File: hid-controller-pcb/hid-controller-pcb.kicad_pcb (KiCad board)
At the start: 2 copper layers, 16 parts, among them IC1 RT9080-33GJ5, J1 10118194-0011LF, U1 STM32F103C8Tx, U2 32.768KHz, U3 COM-09032, U4 COM-09032, Y1 8MHz

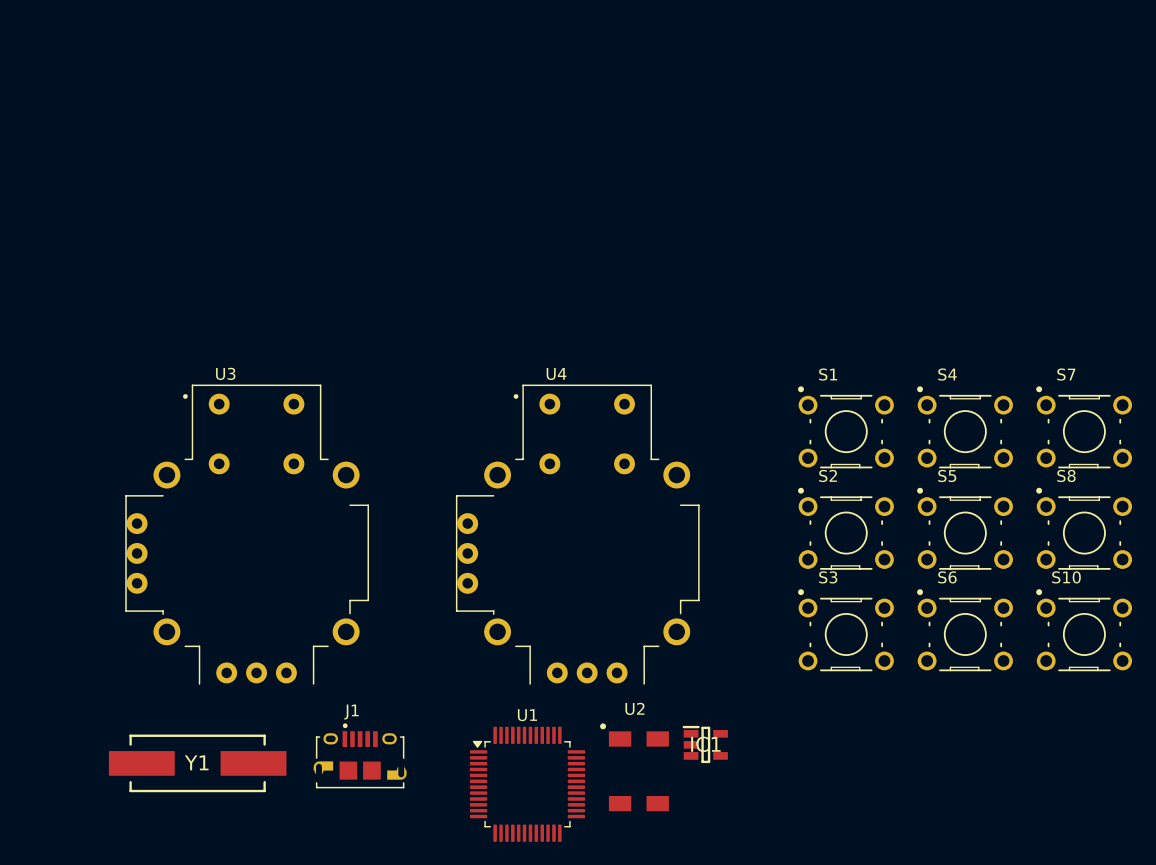
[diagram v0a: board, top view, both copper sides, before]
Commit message: schematic finished? now onto layout
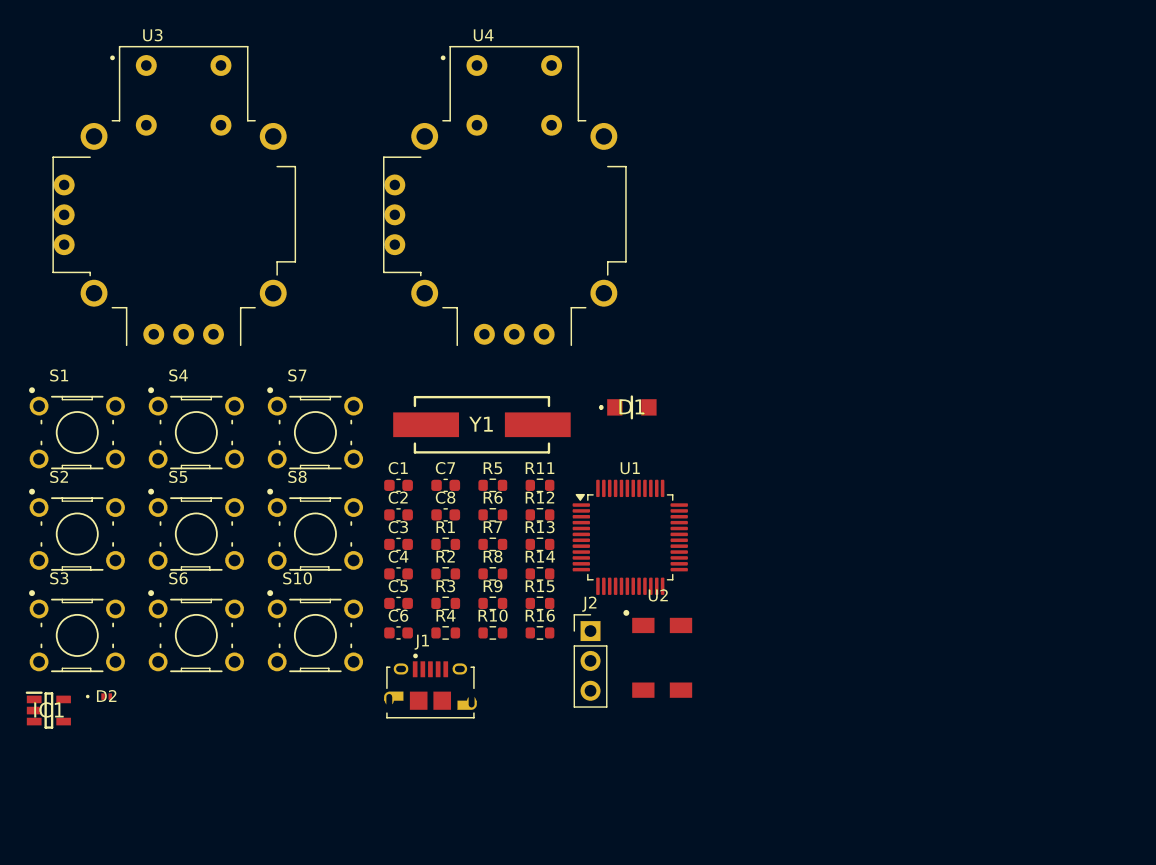
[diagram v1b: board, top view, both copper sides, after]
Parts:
- added C1: 4.7uF, Capacitor_SMD:C_0603_1608Metric, F.Cu at (114.9, 100.6)
- added C2: 26pF, Capacitor_SMD:C_0603_1608Metric, F.Cu at (114.9, 103.1)
- added C3: 26pF, Capacitor_SMD:C_0603_1608Metric, F.Cu at (114.9, 105.7)
- added C4: 8pF, Capacitor_SMD:C_0603_1608Metric, F.Cu at (114.9, 108.2)
- added C5: 8pF, Capacitor_SMD:C_0603_1608Metric, F.Cu at (114.9, 110.7)
- added C6: 0.1uF, Capacitor_SMD:C_0603_1608Metric, F.Cu at (114.9, 113.2)
- added C7: 0.1uF, Capacitor_SMD:C_0603_1608Metric, F.Cu at (118.9, 100.6)
- added C8: 2.2uF, Capacitor_SMD:C_0603_1608Metric, F.Cu at (118.9, 103.1)
- added D1: 3.4V, lib:SMFA2005CA, F.Cu at (134.7, 94.0)
- added D2: 6V, lib:DIODE_VESD05A1B-HD1-GS08_VIS, F.Cu at (90.1, 118.6)
- added J2: Jumper, Connector_PinHeader_2.54mm:PinHeader_1x03_P2.54mm_Vertical, F.Cu at (131.2, 113.0)
- added R1: 22R, Resistor_SMD:R_0603_1608Metric, F.Cu at (118.9, 105.7)
- added R10: 20kR, Resistor_SMD:R_0603_1608Metric, F.Cu at (122.9, 113.2)
- added R11: 20kR, Resistor_SMD:R_0603_1608Metric, F.Cu at (126.9, 100.6)
- added R12: 20kR, Resistor_SMD:R_0603_1608Metric, F.Cu at (126.9, 103.1)
- added R13: 20kR, Resistor_SMD:R_0603_1608Metric, F.Cu at (126.9, 105.7)
- added R14: 20kR, Resistor_SMD:R_0603_1608Metric, F.Cu at (126.9, 108.2)
- added R15: 20kR, Resistor_SMD:R_0603_1608Metric, F.Cu at (126.9, 110.7)
- added R16: 20kR, Resistor_SMD:R_0603_1608Metric, F.Cu at (126.9, 113.2)
- added R2: 22R, Resistor_SMD:R_0603_1608Metric, F.Cu at (118.9, 108.2)
- added R3: 1.5kR, Resistor_SMD:R_0603_1608Metric, F.Cu at (118.9, 110.7)
- added R4: 1.5kR, Resistor_SMD:R_0603_1608Metric, F.Cu at (118.9, 113.2)
- added R5: 68kR, Resistor_SMD:R_0603_1608Metric, F.Cu at (122.9, 100.6)
- added R6: 13kR, Resistor_SMD:R_0603_1608Metric, F.Cu at (122.9, 103.1)
- added R7: 1.5kR, Resistor_SMD:R_0603_1608Metric, F.Cu at (122.9, 105.7)
- added R8: 1.5kR, Resistor_SMD:R_0603_1608Metric, F.Cu at (122.9, 108.2)
- added R9: 20kR, Resistor_SMD:R_0603_1608Metric, F.Cu at (122.9, 110.7)
- moved S1 65.4 mm to (87.6, 96.1)
- moved S10 65.4 mm to (107.8, 113.4)
- moved S2 65.4 mm to (87.6, 104.8)
- moved S3 65.4 mm to (87.6, 113.4)
- moved S7 65.4 mm to (107.8, 96.1)
- moved S8 65.4 mm to (107.8, 104.8)
- moved S4 65.4 mm to (97.7, 96.1)
- moved S5 65.4 mm to (97.7, 104.8)
- moved S6 65.4 mm to (97.7, 113.4)
- moved IC1 55.9 mm to (85.2, 119.8)
- moved Y1 37.6 mm to (122.0, 95.5)
- moved U3 29.5 mm to (96.6, 77.6)
- moved U4 29.5 mm to (124.7, 77.6)
- moved U1 22.7 mm to (134.6, 105.1)
- moved U2 9.85 mm to (137.3, 115.3)
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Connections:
- U1 pad 16: unconnected-(U1-PA6-Pad16) -> DPAD_1
- U1 pad 17: unconnected-(U1-PA7-Pad17) -> DPAD_2
- U1 pad 29: unconnected-(U1-PA8-Pad29) -> DPAD_3
- U1 pad 30: unconnected-(U1-PA9-Pad30) -> DPAD_4
- U1 pad 34: unconnected-(U1-PA13-Pad34) -> SWDIO
- U1 pad 37: unconnected-(U1-PA14-Pad37) -> SWCLK
- U1 pad 42: unconnected-(U1-PB6-Pad42) -> BTN_1
- U1 pad 43: unconnected-(U1-PB7-Pad43) -> BTN_2
- U1 pad 45: unconnected-(U1-PB8-Pad45) -> BTN_3
- U1 pad 46: unconnected-(U1-PB9-Pad46) -> BTN_4
